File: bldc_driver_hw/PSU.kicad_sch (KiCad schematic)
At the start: 26 parts, among them U1 AMS1117-3.3, U2 TPS54260DGQ

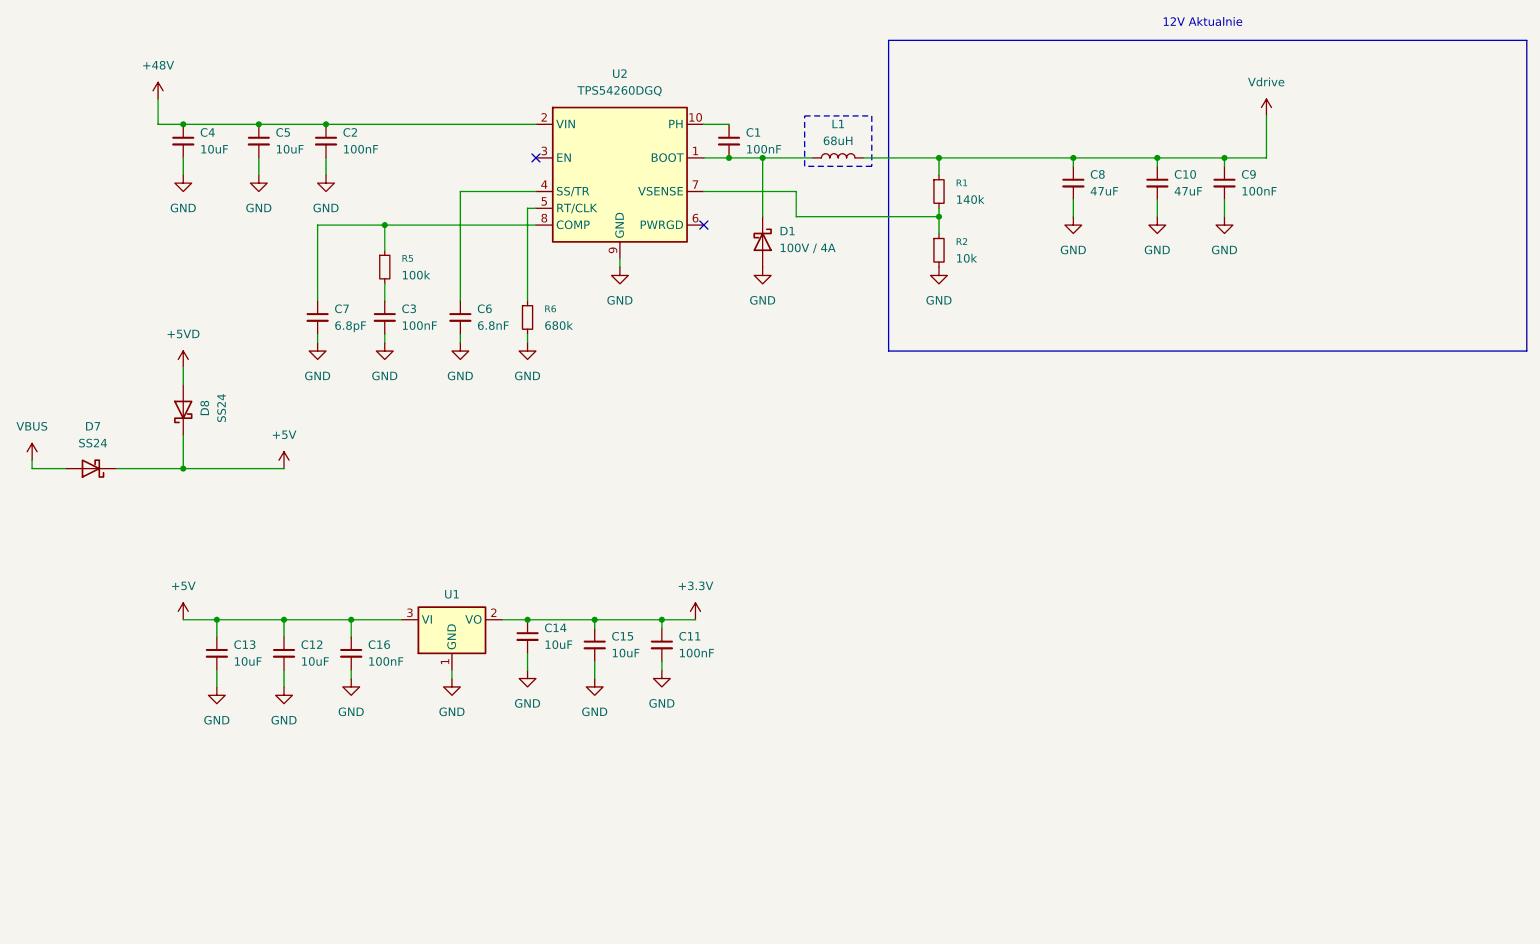
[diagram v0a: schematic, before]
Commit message: wip
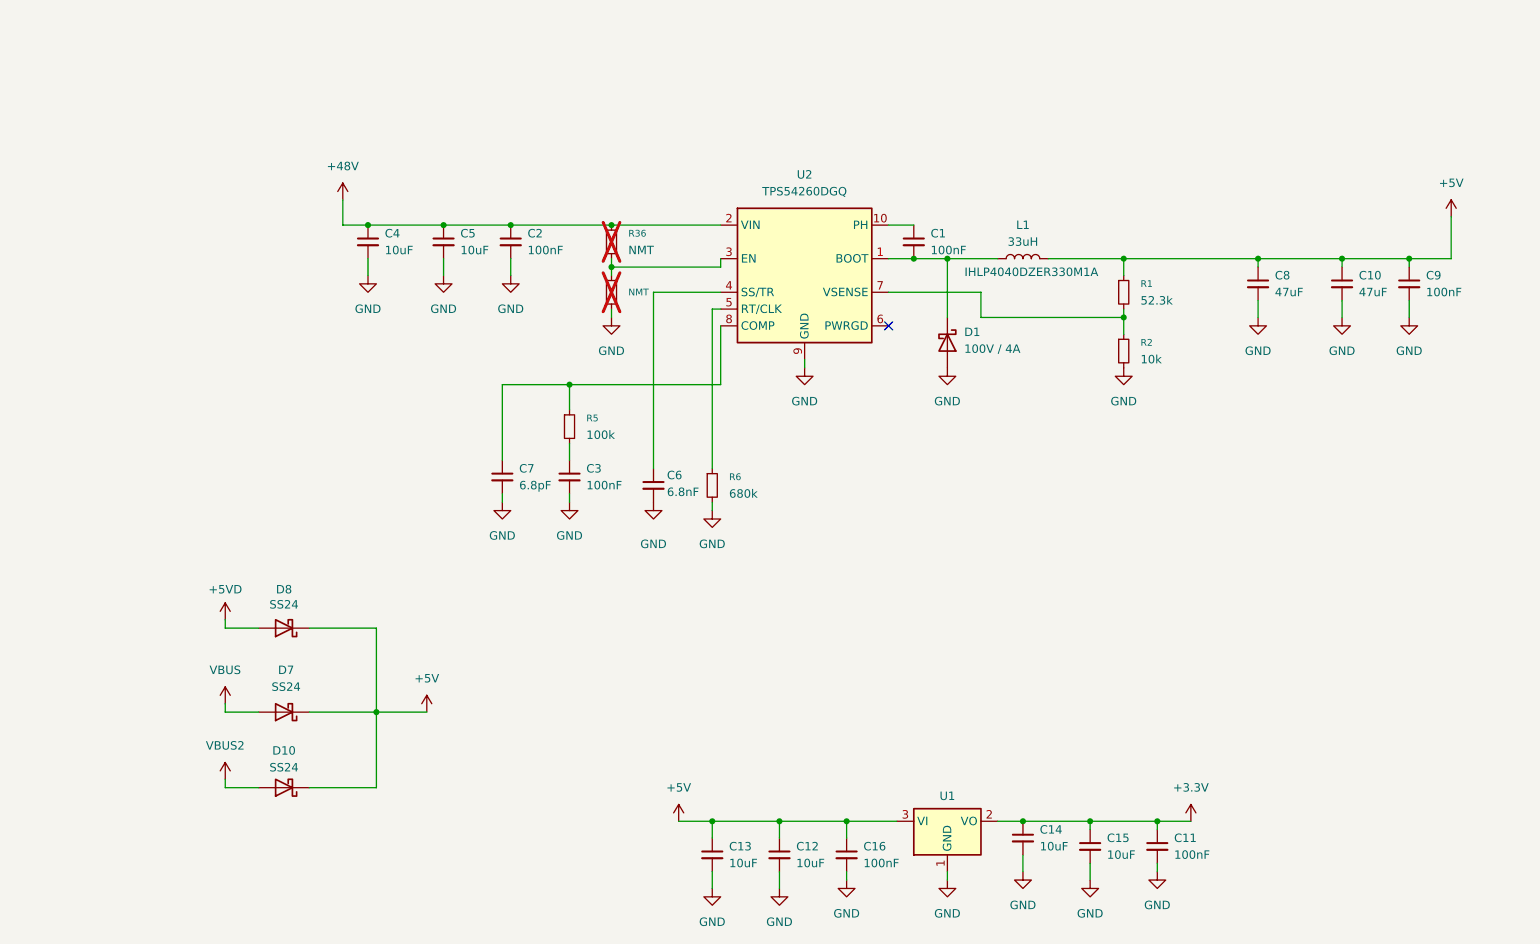
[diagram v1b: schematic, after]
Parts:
- added D10: SS24, Diode_SMD:D_SMA, symbol Diode:SS24
- added NMT: 100k, Resistor_SMD:R_0603_1608Metric_Pad0.98x0.95mm_HandSolder, symbol Device:R_Small
- added R36: NMT, Resistor_SMD:R_0603_1608Metric_Pad0.98x0.95mm_HandSolder, symbol Device:R_Small
- L1: value 68uH -> 33uH; footprint (none) -> Inductor_SMD:L_Vishay_IHLP-4040
- R1: value 140k -> 52.3k
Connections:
- net Vdrive is gone; now on net +5V: C10.1, C8.1, C9.1, L1.2, R1.1
- net +48V: now also R36.1
- net +5V: now also D10.1 (K)
- net GND: now also NMT.2
- net at U2.3 (EN): now also NMT.1, R36.2
- new net VBUS2: D10.2 (A)
- no-connect marks 2 -> 1
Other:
- note removed: "12V Aktualnie"
- moved on the sheet: C1, C10, C11, C12, C13, C14, C15, C16, C2, C3, C4, C5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
